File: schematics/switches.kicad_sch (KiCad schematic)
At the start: 5 parts, among them Q1 NMOS

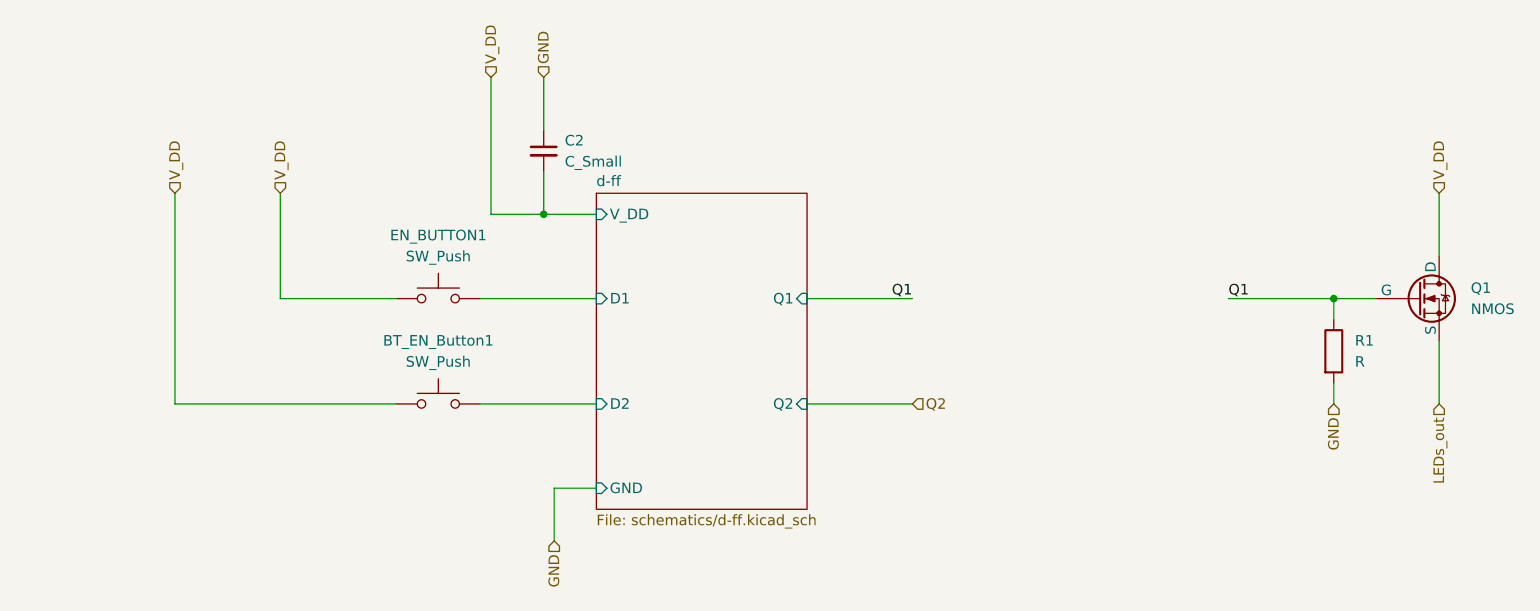
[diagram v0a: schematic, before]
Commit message: 15.11.2025 16:38
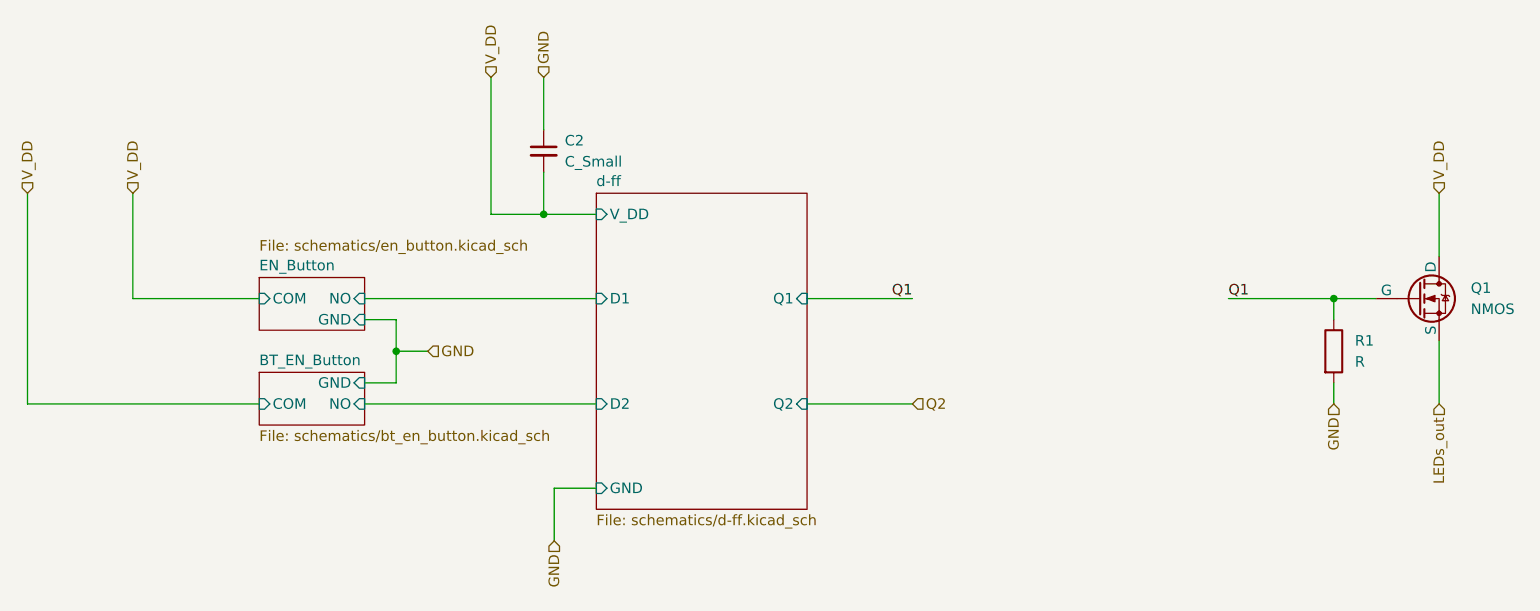
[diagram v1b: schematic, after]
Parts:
- removed BT_EN_Button1, EN_BUTTON1: SW_Push, symbol Switch:SW_Push
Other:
- added sheet BT_EN_Button (schematics/bt_en_button.kicad_sch)
- added sheet EN_Button (schematics/en_button.kicad_sch)
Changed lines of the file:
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@@
 		(color 0 0 0 0)
 	)
-	(wire
-		(pts
-			(xy 50.8 101.6) (xy 77.47 101.6)
+	(junction
+		(at 77.47 95.25)
+		(diameter 0)
+		(color 0 0 0 0)
+	)
+	(wire
+		(pts
+			(xy 33.02 101.6) (xy 60.96 101.6)
 		)
 		(stroke
@@
 	(wire
 		(pts
-			(xy 77.47 88.9) (xy 63.5 88.9)
-		)
-		(stroke
-			(width 0)
-			(type default)
-		)
-	)
-	(wire
-		(pts
-			(xy 87.63 88.9) (xy 101.6 88.9)
+			(xy 45.72 88.9) (xy 60.96 88.9)
 		)
 		(stroke
@@
 	(wire
 		(pts
+			(xy 77.47 99.06) (xy 77.47 95.25)
+		)
+		(stroke
+			(width 0)
+			(type default)
+		)
+	)
+	(wire
+		(pts
 			(xy 177.8 88.9) (xy 190.5 88.9)
 		)
@@
 	(wire
 		(pts
-			(xy 63.5 88.9) (xy 63.5 76.2)
+			(xy 73.66 99.06) (xy 77.47 99.06)
+		)
+		(stroke
+			(width 0)
+			(type default)
+		)
+	)
+	(wire
+		(pts
+			(xy 45.72 88.9) (xy 45.72 76.2)
+		)
+		(stroke
+			(width 0)
+			(type default)
+		)
+	)
+	(wire
+		(pts
+			(xy 73.66 91.44) (xy 77.47 91.44)
 		)
 		(stroke
@@
 	(wire
 		(pts
+			(xy 73.66 88.9) (xy 101.6 88.9)
+		)
+		(stroke
+			(width 0)
+			(type default)
+		)
+	)
+	(wire
+		(pts
 			(xy 96.52 111.76) (xy 101.6 111.76)
 		)
@@
 	(wire
 		(pts
-			(xy 87.63 101.6) (xy 101.6 101.6)
+			(xy 73.66 101.6) (xy 101.6 101.6)
 		)
 		(stroke
@@
 	(wire
 		(pts
-			(xy 50.8 76.2) (xy 50.8 101.6)
+			(xy 33.02 76.2) (xy 33.02 101.6)
 		)
 		(stroke
@@
 	(wire
 		(pts
+			(xy 77.47 95.25) (xy 81.28 95.25)
+		)
+		(stroke
+			(width 0)
+			(type default)
+		)
+	)
+	(wire
+		(pts
 			(xy 88.9 78.74) (xy 95.25 78.74)
+		)
+		(stroke
+			(width 0)
+			(type default)
+		)
+	)
+	(wire
+		(pts
+			(xy 77.47 91.44) (xy 77.47 95.25)
 		)
 		(stroke
@@
 	(hierarchical_label "V_DD"
 		(shape input)
-		(at 50.8 76.2 90)
+		(at 33.02 76.2 90)
 		(effects
 			(font
@@
 	(hierarchical_label "GND"
 		(shape input)
+		(at 81.28 95.25 0)
+		(effects
+			(font
+				(size 1.27 1.27)
+			)
+			(justify left)
+		)
+	)
+	(hierarchical_label "GND"
+		(shape input)
 		(at 190.5 101.6 270)
 		(effects
@@
 	(hierarchical_label "V_DD"
 		(shape input)
-		(at 63.5 76.2 90)
+		(at 45.72 76.2 90)
 		(effects
 			(font
@@
 	)
 	(symbol
-		(lib_id "Switch:SW_Push")
-		(at 82.55 88.9 0)
-		(unit 1)
-		(exclude_from_sim no)
-		(in_bom yes)
-		(on_board yes)
-		(dnp no)
-		(fields_autoplaced yes)
-		(property "Reference" "EN_BUTTON1"
-			(at 82.55 81.28 0)
-			(effects
-				(font
-					(size 1.27 1.27)
-				)
-			)
-		)
-		(property "Value" "SW_Push"
-			(at 82.55 83.82 0)
-			(effects
-				(font
-					(size 1.27 1.27)
-				)
-			)
-		)
-		(property "Footprint" ""
-			(at 82.55 83.82 0)
-			(effects
-				(font
-					(size 1.27 1.27)
-				)
-				(hide yes)
-			)
-		)
-		(property "Datasheet" "~"
-			(at 82.55 83.82 0)
-			(effects
-				(font
-					(size 1.27 1.27)
-				)
-				(hide yes)
-			)
-		)
-		(property "Description" "Push button switch, generic, two pins"
-			(at 82.55 88.9 0)
-			(effects
-				(font
-					(size 1.27 1.27)
-				)
-				(hide yes)
-			)
-		)
-		(pin "2"
-		)
-		(pin "1"
-		)
-		(instances
-			(project ""
-				(path "/d9fee8f2-a86d-4098-a09f-80e037052314/8f5105e1-dc63-457a-99c7-3c491c0ccd8f"
-					(reference "EN_BUTTON1")
-					(unit 1)
-				)
-			)
-		)
-	)
-	(symbol
-		(lib_id "Switch:SW_Push")
-		(at 82.55 101.6 0)
-		(unit 1)
-		(exclude_from_sim no)
-		(in_bom yes)
-		(on_board yes)
-		(dnp no)
-		(fields_autoplaced yes)
-		(property "Reference" "BT_EN_Button1"
-			(at 82.55 93.98 0)
-			(effects
-				(font
-					(size 1.27 1.27)
-				)
-			)
-		)
-		(property "Value" "SW_Push"
-			(at 82.55 96.52 0)
-			(effects
-				(font
-					(size 1.27 1.27)
-				)
-			)
-		)
-		(property "Footprint" ""
-			(at 82.55 96.52 0)
-			(effects
-				(font
-					(size 1.27 1.27)
-				)
-				(hide yes)
-			)
-		)
-		(property "Datasheet" "~"
-			(at 82.55 96.52 0)
-			(effects
-				(font
-					(size 1.27 1.27)
-				)
-				(hide yes)
-			)
-		)
-		(property "Description" "Push button switch, generic, two pins"
-			(at 82.55 101.6 0)
-			(effects
-				(font
-					(size 1.27 1.27)
-				)
-				(hide yes)
-			)
-		)
-		(pin "2"
-		)
-		(pin "1"
-		)
-		(instances
-			(project "ruecklicht"
-				(path "/d9fee8f2-a86d-4098-a09f-80e037052314/8f5105e1-dc63-457a-99c7-3c491c0ccd8f"
-					(reference "BT_EN_Button1")
-					(unit 1)
-				)
-			)
-		)
-	)
-	(symbol
 		(lib_id "Device:R")
 		(at 190.5 95.25 0)
@@
 	)
 	(sheet
+		(at 60.96 86.36)
+		(size 12.7 6.35)
+		(exclude_from_sim no)
+		(in_bom yes)
+		(on_board yes)
+		(dnp no)
+		(stroke
+			(width 0.1524)
+			(type solid)
+		)
+		(fill
+			(color 0 0 0 0.0000)
+		)
+		(property "Sheetname" "EN_Button"
+			(at 60.96 85.6484 0)
+			(effects
+				(font
+					(size 1.27 1.27)
+				)
+				(justify left bottom)
+			)
+		)
+		(property "Sheetfile" "schematics/en_button.kicad_sch"
+			(at 60.96 81.788 0)
+			(effects
+				(font
+					(size 1.27 1.27)
+				)
+				(justify left top)
+			)
+		)
+		(property "Field2" ""
+			(at 60.96 86.36 0)
+			(effects
+				(font
+					(size 1.27 1.27)
+				)
+			)
+		)
+		(pin "COM" input
+			(at 60.96 88.9 180)
+			(effects
+				(font
+					(size 1.27 1.27)
+				)
+				(justify left)
+			)
+		)
+		(pin "GND" input
+			(at 73.66 91.44 0)
+			(effects
+				(font
+					(size 1.27 1.27)
+				)
+				(justify right)
+			)
+		)
+		(pin "NO" input
+			(at 73.66 88.9 0)
+			(effects
+				(font
+					(size 1.27 1.27)
+				)
+				(justify right)
+			)
+		)
+		(instances
+			(project "ruecklicht"
+				(path "/d9fee8f2-a86d-4098-a09f-80e037052314/8f5105e1-dc63-457a-99c7-3c491c0ccd8f"
+					(page "11")
+				)
+			)
+		)
+	)
+	(sheet
 		(at 101.6 76.2)
 		(size 25.4 38.1)
@@
 				)
 			)
+		)
+	)
+	(sheet
+		(at 60.96 97.79)
+		(size 12.7 6.35)
+		(exclude_from_sim no)
+		(in_bom yes)
+		(on_board yes)
+		(dnp no)
+		(fields_autoplaced yes)
+		(stroke
+			(width 0.1524)
+			(type solid)
+		)
+		(fill
+			(color 0 0 0 0.0000)
+		)
+		(property "Sheetname" "BT_EN_Button"
+			(at 60.96 97.0784 0)
+			(effects
+				(font
+					(size 1.27 1.27)
+				)
+				(justify left bottom)
+			)
+		)
+		(property "Sheetfile" "schematics/bt_en_button.kicad_sch"
+			(at 60.96 104.7246 0)
+			(effects
+				(font
+					(size 1.27 1.27)
+				)
+				(justify left top)
+			)
+		)
+		(property "Field2" ""
+			(at 60.96 97.79 0)
+			(effects
+				(font
+					(size 1.27 1.27)
+				)
+			)
+		)
+		(pin "COM" input
+			(at 60.96 101.6 180)
+			(effects
+				(font
+					(size 1.27 1.27)
+				)
+				(justify left)
+			)
+		)
+		(pin "GND" input
+			(at 73.66 99.06 0)
+			(effects
+				(font
+					(size 1.27 1.27)
+				)
+				(justify right)
+			)
+		)
+		(pin "NO" input
+			(at 73.66 101.6 0)
+			(effects
+				(font
+					(size 1.27 1.27)
+				)
+				(justify right)
+			)
+		)
+		(instances
+			(project "ruecklicht"
+				(path "/d9fee8f2-a86d-4098-a09f-80e037052314/8f5105e1-dc63-457a-99c7-3c491c0ccd8f"
+					(page "10")
+				)
+			)

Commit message: 16.11.2025 16:28 -> began with pcb
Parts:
- Q1: footprint Package_TO_SOT_SMD:TO-252-3_TabPin2 -> footprints:mosfet
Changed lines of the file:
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@@
 			)
 		)
-		(property "Footprint" "Package_TO_SOT_SMD:TO-252-3_TabPin2"
+		(property "Footprint" "footprints:mosfet"
 			(at 205.74 86.36 0)
 			(effects
@@
 			)
 		)
-		(property "Sim.Pins" "1=D 2=G 3=S"
+		(property "Sim.Pins" "1=G 2=D 3=S"
 			(at 200.66 104.14 0)
 			(effects
